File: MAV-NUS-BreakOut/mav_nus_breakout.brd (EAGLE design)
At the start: 8.7 x 13.3 mm, 37 parts

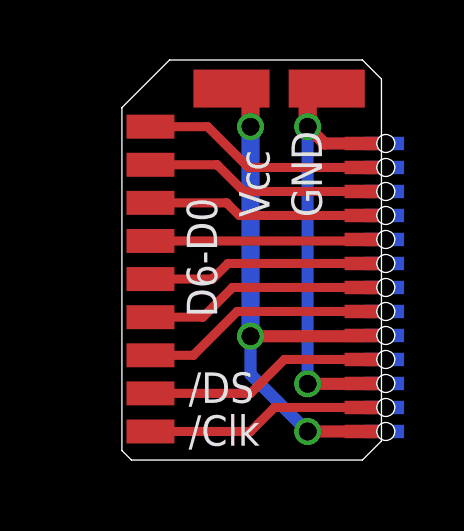
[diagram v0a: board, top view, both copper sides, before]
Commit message: update adapter PCB
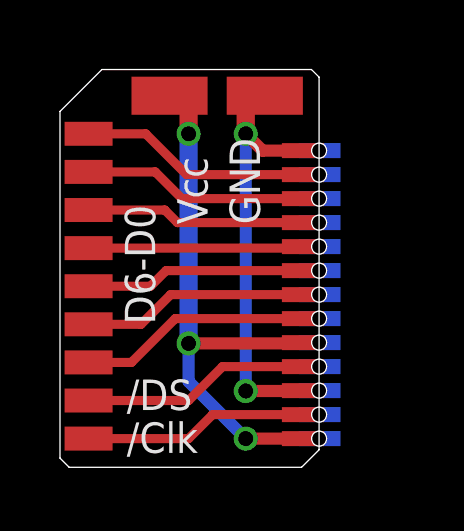
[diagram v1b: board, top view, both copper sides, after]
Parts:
- removed PAD1, PAD2: (no value), wirepad:SMD1,27-2,54
- removed U$1, U$10, U$11, U$12, U$13, U$2, U$23, U$24, U$25, U$26, U$27, U$28, U$29, U$3, U$30, U$31, U$32, U$33, U$34, U$35, U$4, U$5, U$6, U$7, U$8, U$9: SMD0,45, wirepad:SMD0,45-1,35
- removed U$14, U$15, U$16, U$17, U$18, U$19, U$20, U$21, U$22: SMD1, wirepad:SMD0,8-1,6
- added PAD13, PAD14: (no value), wirepad:SMD1,27-2,54
- added U$211, U$212, U$213, U$214, U$215, U$222, U$226, U$227, U$228, U$229, U$230, U$231, U$232, U$233, U$234, U$235, U$236, U$237, U$238, U$239, U$240, U$241, U$242, U$243, U$244, U$245: SMD0,45, wirepad:SMD0,5-1,4
- added U$216, U$217, U$218, U$219, U$220, U$221, U$223, U$224, U$225: SMD1, wirepad:SMD0,8-1,6
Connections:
- removed net N$1: U$1.P$1, U$14.P$1
- removed net N$10: PAD1.1, U$10.P$1, U$11.P$1
- removed net N$11: PAD2.1, U$12.P$1, U$13.P$1
- removed net N$2: U$15.P$1, U$2.P$1
- removed net N$3: U$16.P$1, U$3.P$1
- removed net N$4: U$17.P$1, U$4.P$1
- removed net N$5: U$18.P$1, U$5.P$1
- removed net N$6: U$19.P$1, U$6.P$1
- removed net N$7: U$20.P$1, U$7.P$1
- removed net N$8: U$21.P$1, U$8.P$1
- removed net N$9: U$22.P$1, U$9.P$1
- new net N$67: U$211.P$1, U$216.P$1
- new net N$68: U$217.P$1, U$222.P$1
- new net N$69: U$218.P$1, U$226.P$1
- new net N$70: U$219.P$1, U$227.P$1
- new net N$71: U$220.P$1, U$228.P$1
- new net N$72: U$221.P$1, U$229.P$1
- new net N$73: U$223.P$1, U$230.P$1
- new net N$74: U$224.P$1, U$231.P$1
- new net N$75: U$225.P$1, U$232.P$1
- new net N$76: PAD13.1, U$212.P$1, U$213.P$1
- new net N$77: PAD14.1, U$214.P$1, U$215.P$1
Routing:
- net N$10: track 18.6 -> 0.00 mm, vias 3 -> 0
- net N$76: track 0.00 -> 18.6 mm, vias 0 -> 3
- net N$11: track 14.5 -> 0.00 mm, vias 2 -> 0
- net N$77: track 0.00 -> 14.5 mm, vias 0 -> 2
- net N$2: track 7.75 -> 0.00 mm
- net N$68: track 0.00 -> 7.75 mm
- net N$9: track 7.71 -> 0.00 mm
- net N$75: track 0.00 -> 7.71 mm
- net N$69: track 0.00 -> 7.61 mm
- net N$3: track 7.61 -> 0.00 mm
- net N$1: track 7.55 -> 0.00 mm
- net N$67: track 0.00 -> 7.55 mm
- net N$8: track 7.51 -> 0.00 mm
- net N$74: track 0.00 -> 7.51 mm
- net N$70: track 0.00 -> 7.48 mm
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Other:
- board size 8.7 x 13.3 mm -> 8.6 x 13.3 mm
